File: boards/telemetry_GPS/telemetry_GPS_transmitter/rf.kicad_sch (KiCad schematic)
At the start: 10 parts, among them J4 Conn_Coaxial, U4 BALFHB-WL-02D3, U5 MASW-007221, U6 74AHC1G04SE-7

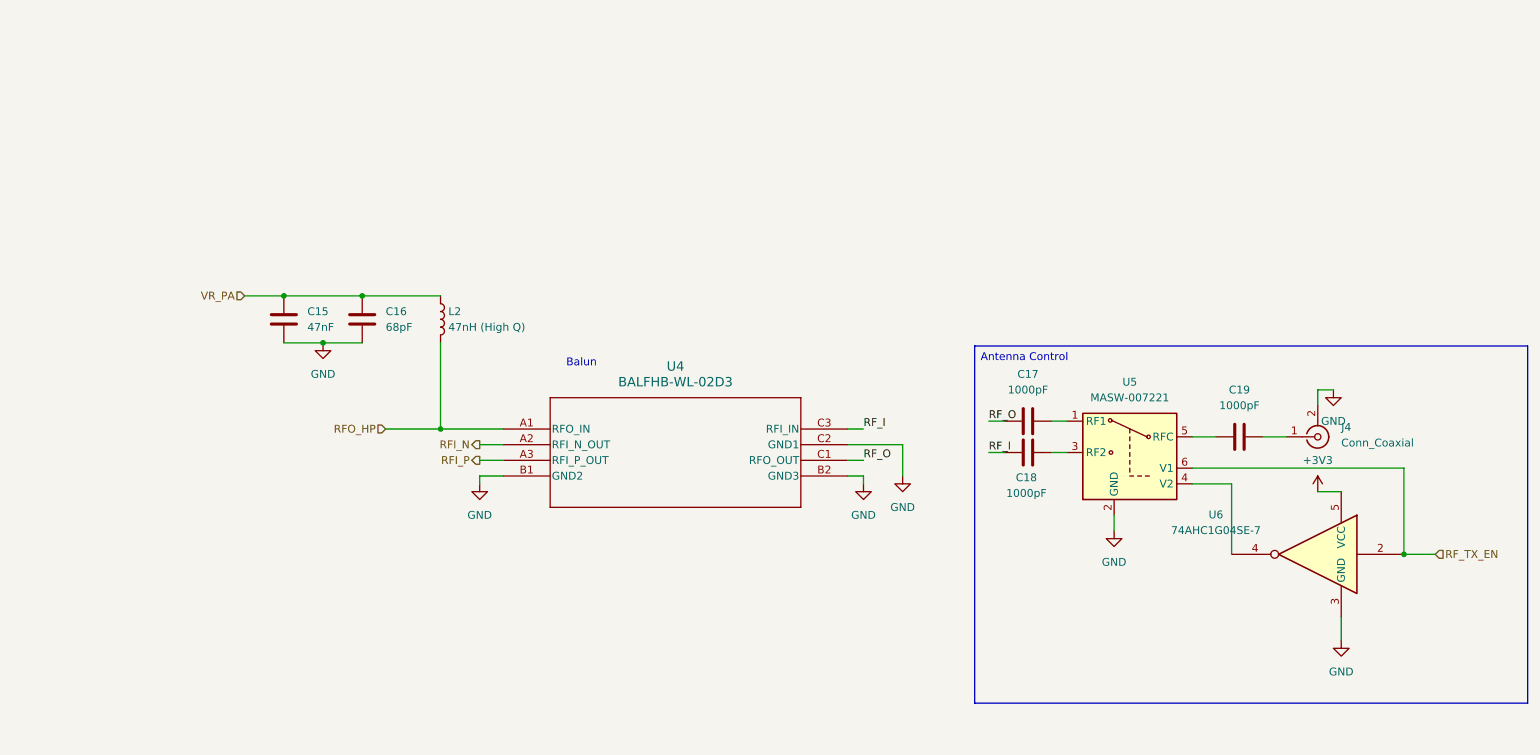
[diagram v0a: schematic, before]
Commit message: Finished Schematic
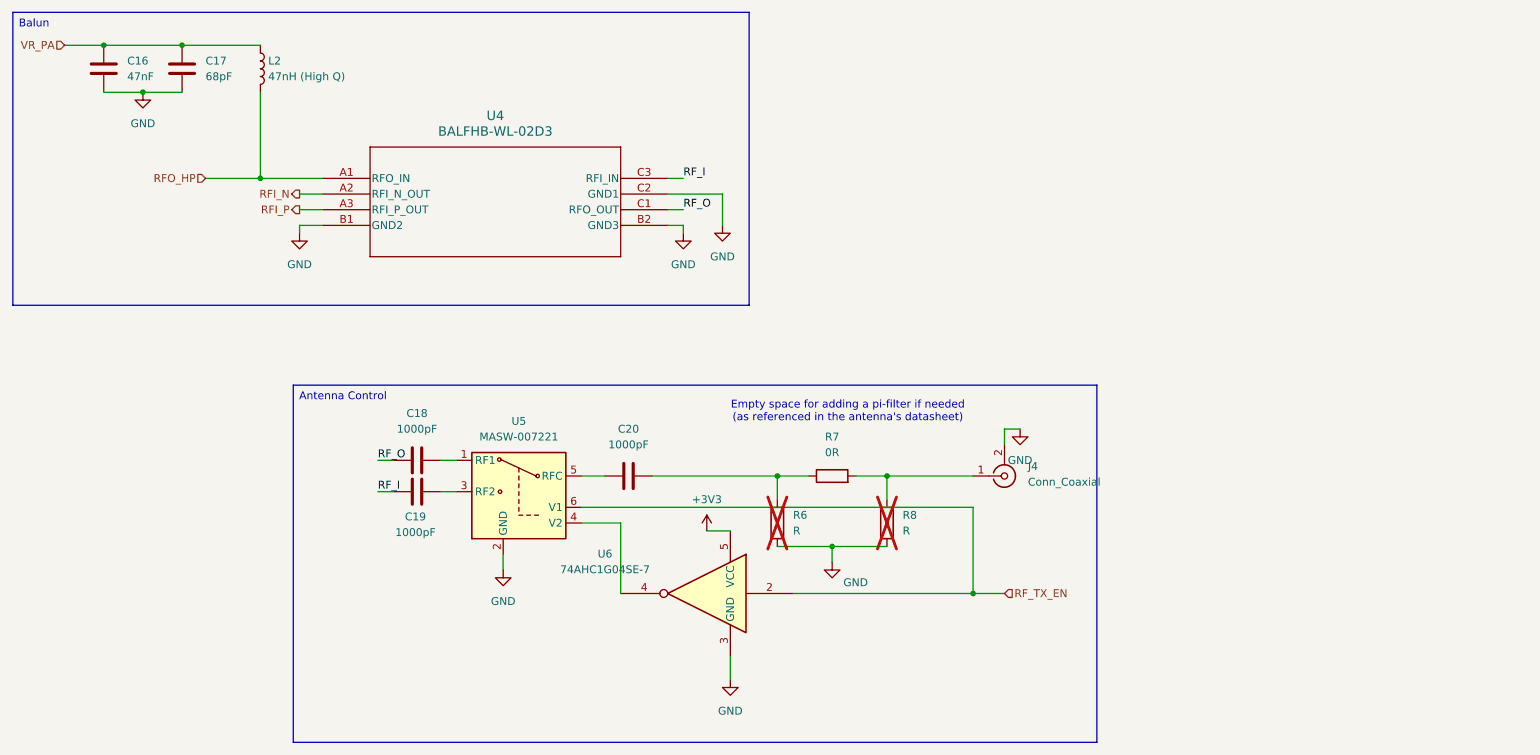
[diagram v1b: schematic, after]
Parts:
- added R6, R8: R, Resistor_SMD:R_0603_1608Metric_Pad0.98x0.95mm_HandSolder, symbol Device:R
- added R7: 0R, Resistor_SMD:R_0603_1608Metric_Pad0.98x0.95mm_HandSolder, symbol Device:R
- renumbered C15 to C16, C16 to C17, C17 to C18, C18 to C19, C19 to C20
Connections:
- net GND: now also R6.2, R8.2
- net at C20.1: now also R6.1, R7.1; no longer J4.1 (In)
- new net: J4.1 (In), R7.2, R8.1
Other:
- note added: "Empty space for adding a pi-filter if needed (as referenced in the antenna's datasheet)"
- note removed: "Balun"
- moved on the sheet: C16, C17, C18, C19, C20, J4, L2, U4, U5, U6
